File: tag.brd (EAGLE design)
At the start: 100 x 80 mm, 9 parts, among them X1 OMAT_IC_PIIKKIRIMA-8A, X2 OMAT_IC_PIIKKIRIMA-8B

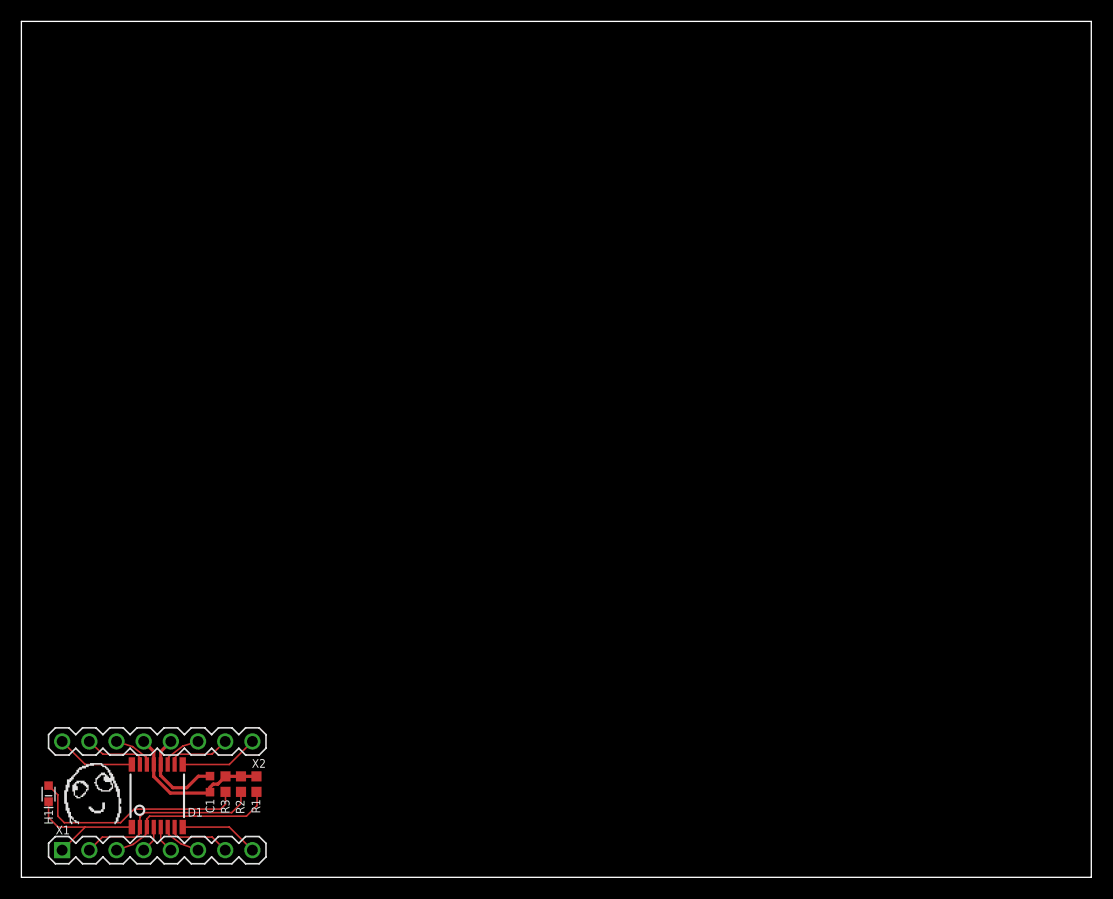
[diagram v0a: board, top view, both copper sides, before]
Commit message: Rounding done... Finished
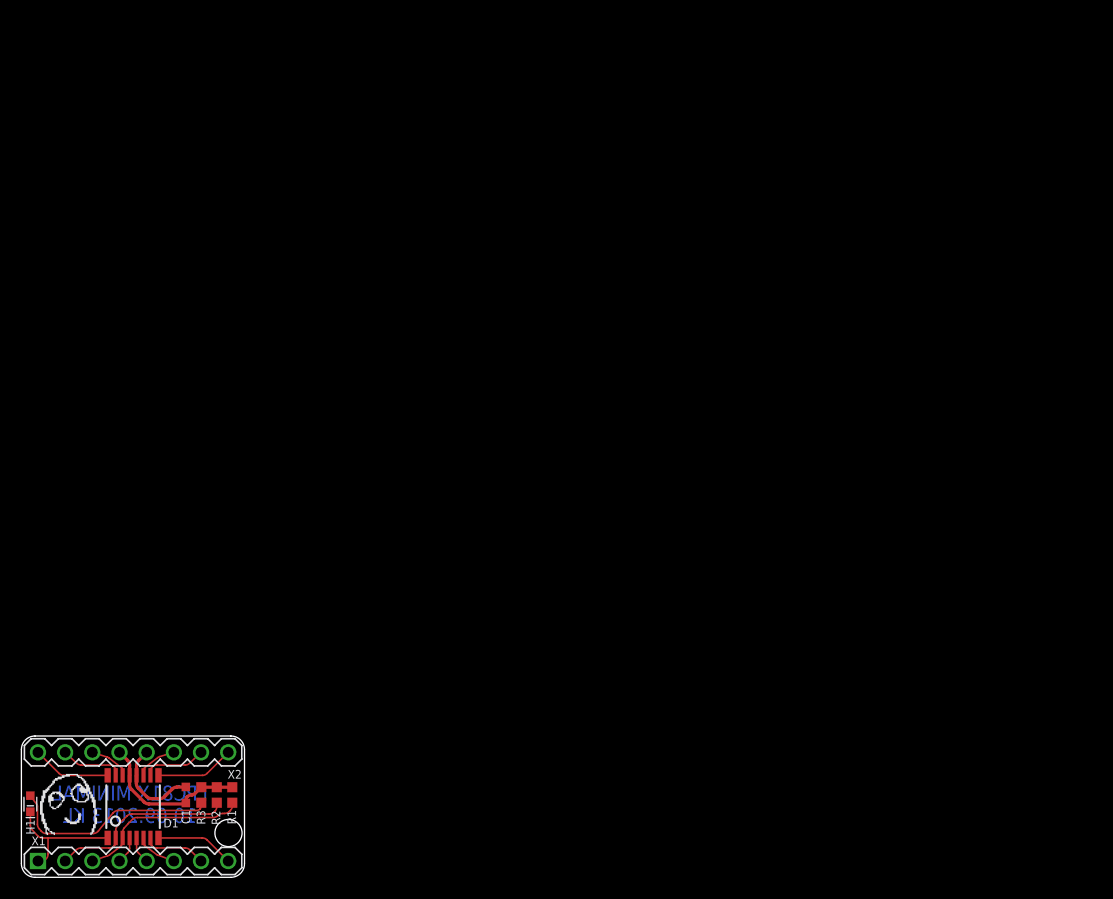
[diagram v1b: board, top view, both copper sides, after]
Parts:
- moved C1 2.48 mm to (15.4, 7.70)
- moved D1 2.48 mm to (10.4, 6.60)
- moved R1 2.48 mm to (19.7, 7.70)
- moved R2 2.48 mm to (18.3, 7.70)
- moved X1 2.48 mm to (1.55, 1.52)
- moved X2 2.48 mm to (19.3, 11.7)
- moved U$1 2.48 mm to (4.60, 6.55)
- moved R3 2.48 mm to (16.8, 7.70)
- moved H1 1.94 mm to (0.84, 6.88)
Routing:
- net N$11: track 21.0 -> 20.1 mm
- net N$8: track 12.7 -> 11.8 mm
- net N$6: track 16.7 -> 16.1 mm
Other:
- board size 100 x 80 mm -> 20.9 x 13.2 mm
- board text added: "LPC81X MINIMAL 10.09.2013 KL"
